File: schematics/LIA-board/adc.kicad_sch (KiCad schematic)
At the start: 2 parts, among them U14 ADS1220xPW, U15 DAC80508

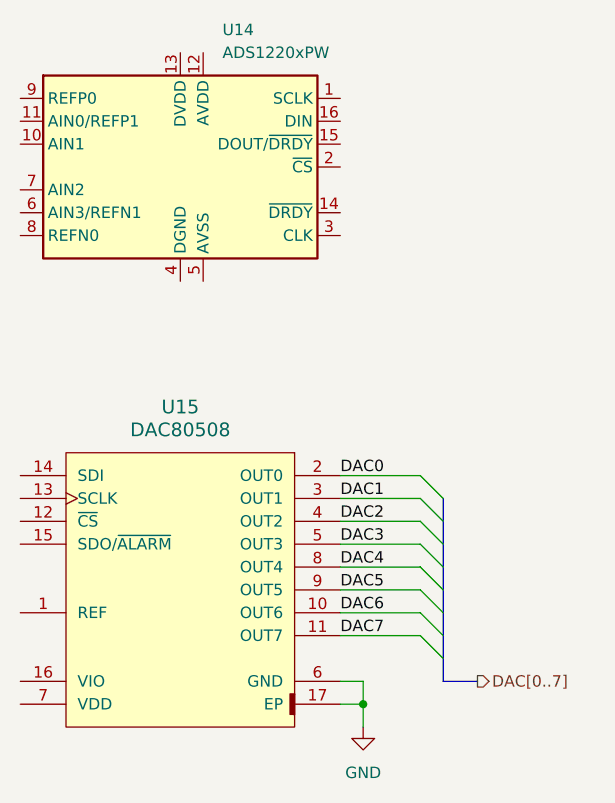
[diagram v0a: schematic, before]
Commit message: modified scematic
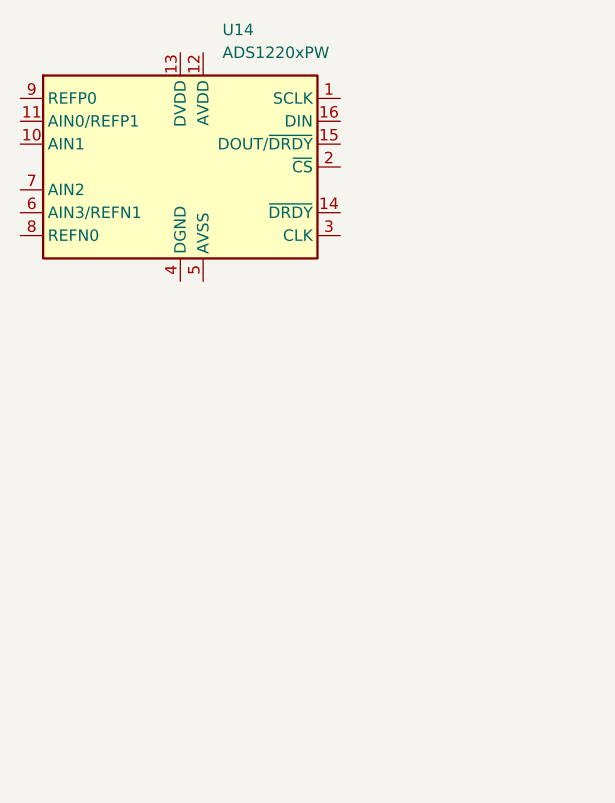
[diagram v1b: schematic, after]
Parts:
- removed U15: DAC80508, Package_SON:Texas_DRX_WSON-10_2.5x2.5mm_P0.5mm, symbol CERN:DAC80508ZRTE
